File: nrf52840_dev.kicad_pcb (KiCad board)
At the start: 2 copper layers, 42.5 x 32 mm, 19 parts, among them J1 SWD, J10 POWER, J2 SPI1, J3 POWER, J4 Conn_01x01, J5 Conn_01x01, J6 SPI2, J7 POWER, J8 Conn_01x01, J9 Conn_01x01

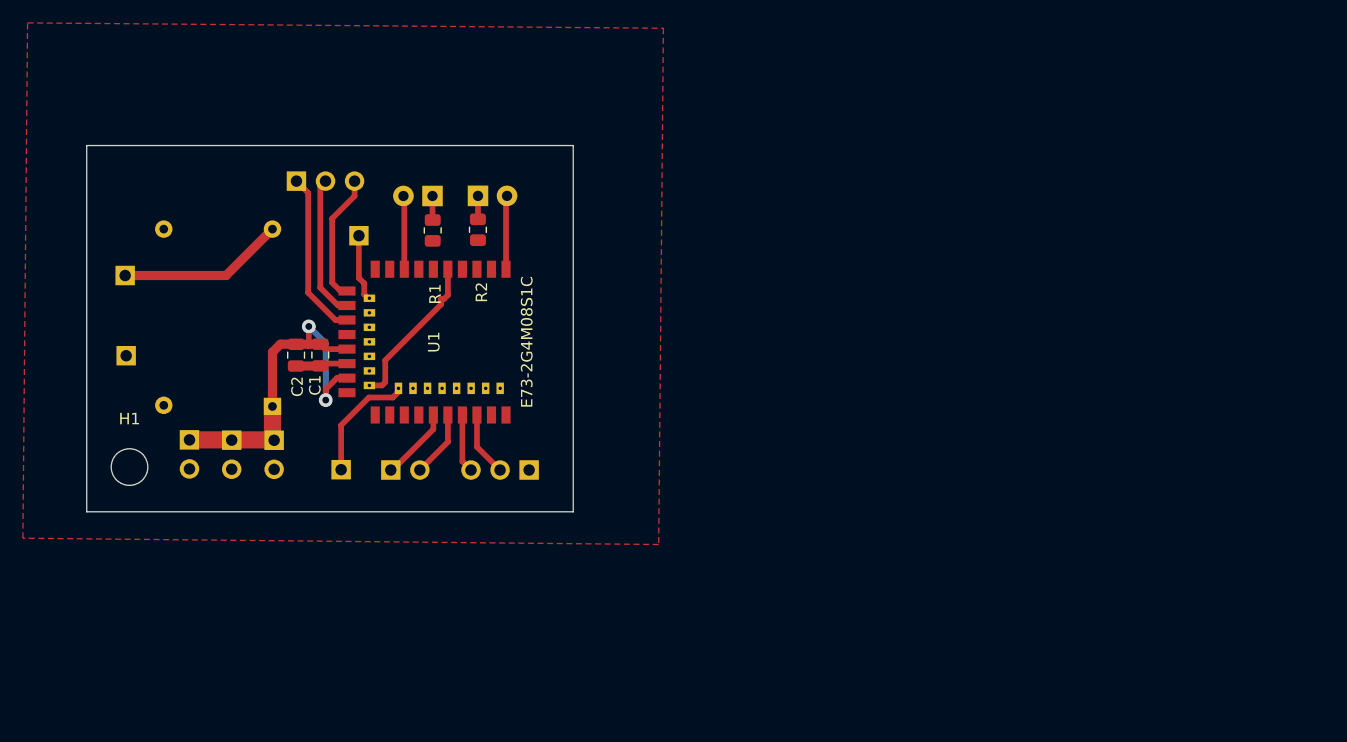
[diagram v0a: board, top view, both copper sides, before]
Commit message: Small fix
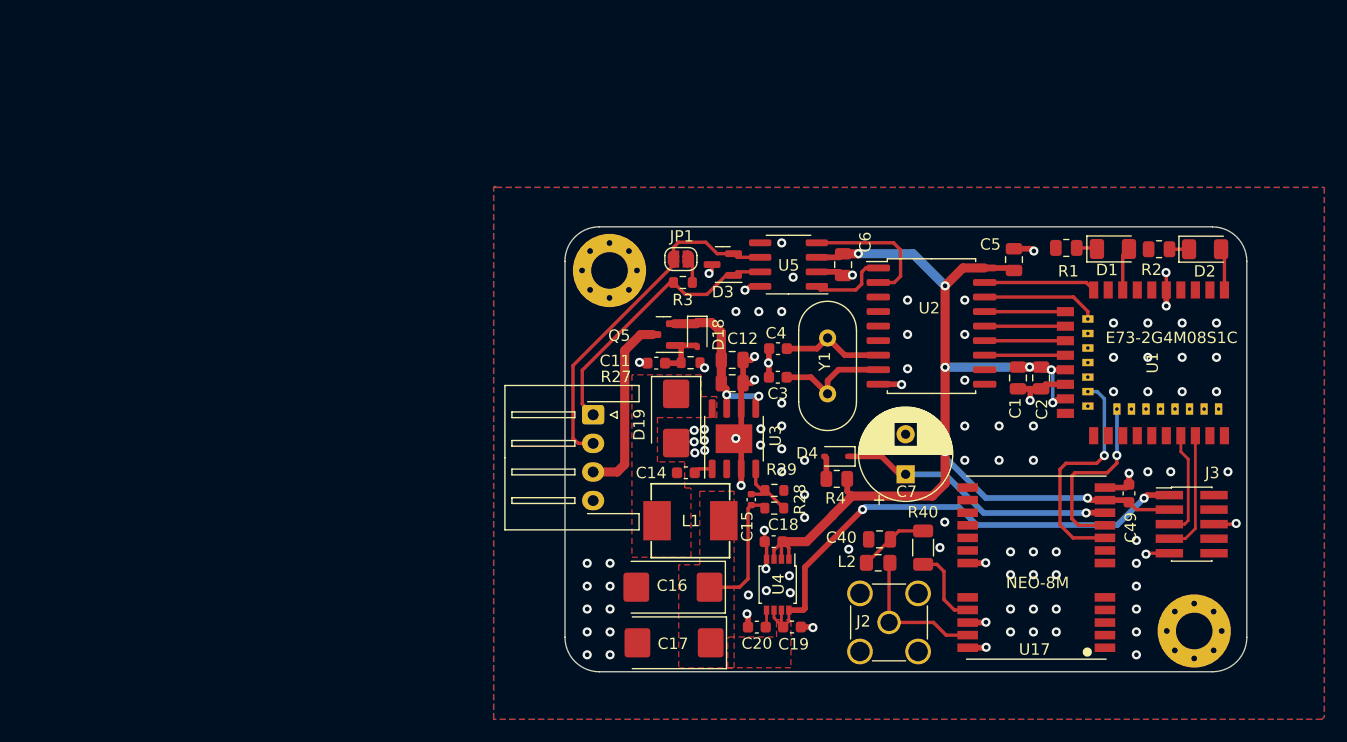
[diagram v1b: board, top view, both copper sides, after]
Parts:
- removed DC1: DC-DC, mini360:DC-DC mini360
- removed J10, J7: POWER, Connector_PinHeader_2.54mm:PinHeader_1x02_P2.54mm_Vertical
- removed J4, J5, J8, J9: Conn_01x01, Connector_PinHeader_2.54mm:PinHeader_1x01_P2.54mm_Vertical
- removed J6: SPI2, Connector_PinHeader_2.54mm:PinHeader_1x02_P2.54mm_Vertical
- added C11: 0.01uF, Capacitor_SMD:C_0603_1608Metric, F.Cu at (128.0, 91.5)
- added C12: 4.7uF, Capacitor_SMD:C_0805_2012Metric, F.Cu at (134.7, 91.2)
- added C13: 0.1uF, Capacitor_SMD:C_0805_2012Metric, F.Cu at (134.7, 93.3)
- added C14: 0.1uF, Capacitor_SMD:C_0603_1608Metric, F.Cu at (130.6, 101.1)
- added C15: 1.6pF, Capacitor_SMD:C_0402_1005Metric, F.Cu at (136.3, 103.4)
- added C16: 47uF, Capacitor_Tantalum_SMD:CP_EIA-7343-31_Kemet-D_Pad2.25x2.55mm_HandSolder, F.Cu at (129.5, 111.1)
- added C17: 47uF, Capacitor_Tantalum_SMD:CP_EIA-7343-31_Kemet-D_Pad2.25x2.55mm_HandSolder, F.Cu at (129.6, 116.0)
- added C18: 1uF, Capacitor_SMD:C_0603_1608Metric, F.Cu at (138.3, 107.1)
- added C19: 1uF, Capacitor_SMD:C_0603_1608Metric, F.Cu at (139.9, 114.6)
- added C20: 0.01uF, Capacitor_SMD:C_0603_1608Metric, F.Cu at (136.8, 114.6)
- added C3: C_Small, Capacitor_SMD:C_0603_1608Metric, F.Cu at (138.7, 92.7)
- added C4: C_Small, Capacitor_SMD:C_0603_1608Metric, F.Cu at (138.7, 90.2)
- added C40: 0.01uF, Capacitor_SMD:C_0805_2012Metric, F.Cu at (147.6, 106.9)
- added C49: 0.1uF, Capacitor_SMD:C_0603_1608Metric, F.Cu at (169.3, 102.9)
- added C5: 0.1uF, Capacitor_SMD:C_0805_2012Metric, F.Cu at (159.3, 82.5)
- added C6: 0.1uF, Capacitor_SMD:C_0805_2012Metric, F.Cu at (144.4, 82.9)
- added C7: 1F, Capacitor_THT:CP_Radial_D8.0mm_P3.50mm, F.Cu at (149.8, 101.2)
- added D18: BZT52C16S, Diode_SMD:D_SOD-323, F.Cu at (131.6, 89.0)
- added D19: STPS2L25, Diode_SMD:D_SMB, F.Cu at (129.8, 96.3)
- added D3: NUP2105L, Package_TO_SOT_SMD:SOT-23, F.Cu at (133.9, 82.9)
- added D4: 1N4148, Diode_SMD:D_SOD-323, F.Cu at (143.8, 99.7)
- added H2: MountingHole_Pad, MountingHole:MountingHole_3.2mm_M3_Pad_Via, F.Cu at (175.1, 114.9)
- added JP1: terminator, Jumper:SolderJumper-2_P1.3mm_Open_RoundedPad1.0x1.5mm, F.Cu at (130.2, 82.4)
- added L1: 8.2uH, power:Inductor8.2, F.Cu at (128.1, 105.3)
- added L2: 27nH, Inductor_SMD:L_0805_2012Metric_Pad1.15x1.40mm_HandSolder, F.Cu at (147.4, 109.0)
- added Q5: AO3401A, Package_TO_SOT_SMD:SOT-23, F.Cu at (128.7, 89.0)
- added R27: 10K, Resistor_SMD:R_0603_1608Metric, F.Cu at (131.0, 91.5)
- added R28: 187K, Resistor_SMD:R_0603_1608Metric, F.Cu at (138.3, 104.2)
- added R29: 60.4K, Resistor_SMD:R_0603_1608Metric, F.Cu at (138.4, 102.6)
- added R3: 120, Resistor_SMD:R_0603_1608Metric, F.Cu at (130.4, 84.5)
- added R4: 100, Resistor_SMD:R_0805_2012Metric, F.Cu at (143.8, 101.6)
- added R40: 10, Resistor_SMD:R_1206_3216Metric, F.Cu at (151.4, 107.6)
- added U17: NEO-8M, ublox:NEO-M8N, F.Cu at (161.2, 109.4)
- added U2: MCP2515-xSO, Package_SO:SOIC-18W_7.5x11.6mm_P1.27mm, F.Cu at (152.1, 88.3)
- added U3: ST1S14PHR_MY, Package_SO:SOIC-8-1EP_3.9x4.9mm_P1.27mm_EP2.514x3.2mm, F.Cu at (134.8, 98.1)
- added U4: NCP3335, Package_SO:OnSemi_Micro8, F.Cu at (138.7, 110.9)
- added U5: SN65HVD230, Package_SO:SOIC-8_3.9x4.9mm_P1.27mm, F.Cu at (139.6, 82.9)
- added Y1: 8Mhz, Crystal:Crystal_HC49-U_Vertical, F.Cu at (143.0, 94.2)
- D1, D2: footprint LED_THT:LED_D5.0mm -> LED_SMD:LED_1206_3216Metric; moved to F.Cu
- H1: value MountingHole -> MountingHole_Pad; footprint MountingHole:MountingHole_3.2mm_M3 -> MountingHole:MountingHole_3.2mm_M3_Pad_Via
- J1: value SWD -> Conn_01x04; footprint Connector_PinHeader_2.54mm:PinHeader_1x03_P2.54mm_Vertical -> Connector_JST:JST_XH_S4B-XH-A-1_1x04_P2.50mm_Horizontal; moved to F.Cu
- J2: value SPI1 -> Conn_Coaxial_Power; footprint Connector_PinHeader_2.54mm:PinHeader_1x03_P2.54mm_Vertical -> Connector_Coaxial:SMA_Amphenol_901-144_Vertical; moved to F.Cu
- J3: value POWER -> SWD; footprint Connector_PinHeader_2.54mm:PinHeader_1x02_P2.54mm_Vertical -> Connector_PinHeader_1.27mm:PinHeader_2x05_P1.27mm_Vertical_SMD; moved to F.Cu
- moved J3 87.9 mm to (174.8, 105.6), turned to 0 degrees
- moved C2 65.1 mm to (161.7, 92.8)
- moved J2 64.6 mm to (148.4, 114.2), turned to 180 degrees
- moved D2 63.7 mm to (176.0, 81.5)
- moved U1 62.8 mm to (163.7, 91.5)
- moved C1 61.0 mm to (159.7, 92.8)
- moved D1 59.6 mm to (167.9, 81.5), turned to 0 degrees
- moved R2 59.6 mm to (172.0, 81.5), turned to 180 degrees
- moved R1 55.4 mm to (163.9, 81.4), turned to 180 degrees
- moved H1 45.3 mm to (124.0, 83.4)
- moved J1 7.39 mm to (122.5, 96.0), turned to -90 degrees
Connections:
- J1 pad 1: GND -> /CANH
- J1 pad 2: /SWD_CLK -> /CANL
- J1 pad 3: /SWD_IO -> /12VIN
- J2 pad 1: /SCK -> /ublox/GPS_RF
- J2 pad 2: /MOSI -> GND
- J3 pad 1: /3V3 -> /5V
- J3 pad 2: GND -> unconnected-(J3-Pin_2-Pad2)
- U1 pad 10: unconnected-(U1-P0.30(AIN6)-Pad10) -> /MCP_RST
- U1 pad 12: /RX -> /CS
- U1 pad 17: unconnected-(U1-P1.09-Pad17) -> /IRQ
- U1 pad 22: unconnected-(U1-P0.07-Pad22) -> /RX
- U1 pad 33: /CS -> unconnected-(U1-P0.13-Pad33)
- U1 pad 35: /IRQ -> unconnected-(U1-P0.24-Pad35)
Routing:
- net /3V3: track 33.9 -> 96.5 mm, vias 2 -> 8
- net /5V: track 0.00 -> 57.2 mm, vias 0 -> 2
- net GND: track 18.0 -> 50.9 mm, vias 0 -> 107
- net /CANL: track 0.00 -> 30.0 mm
- net /CANH: track 0.00 -> 24.3 mm
- net /ublox/GPS_VBAT: track 0.00 -> 23.9 mm, vias 0 -> 1
- net Net-(D18-K): track 0.00 -> 15.4 mm, vias 0 -> 2
- net /RX: track 5.80 -> 20.3 mm, vias 0 -> 1
- net /ublox/GPS_RF: track 0.00 -> 12.6 mm
- net Net-(U2-RXCAN): track 0.00 -> 12.1 mm
- net Net-(U2-OSC1): track 0.00 -> 10.2 mm
- net /MCP_RST: track 0.00 -> 9.79 mm
- net Net-(U2-OSC2): track 0.00 -> 8.99 mm
- net /SCK: track 14.6 -> 7.05 mm
- net Net-(U17-VCC_RF): track 0.00 -> 6.98 mm
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- added copper zone on F.Cu, net /5V
- added copper zone on B.Cu, net GND
- added copper zone on F.Cu, net Net-(D19-K)
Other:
- board size 42.5 x 32 mm -> 59.6 x 38.9 mm
- board text added: "12V"
- board text added: "CAN HI"
- board text added: "CAN LOW"
- board text added: "GND"
